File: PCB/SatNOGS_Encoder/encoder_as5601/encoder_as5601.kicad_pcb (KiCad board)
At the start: 2 copper layers, 25.4 x 25.4 mm, 12 parts, among them P1 CONN_02X05, Q1 Q_NMOS_GSD, U1 AS5601

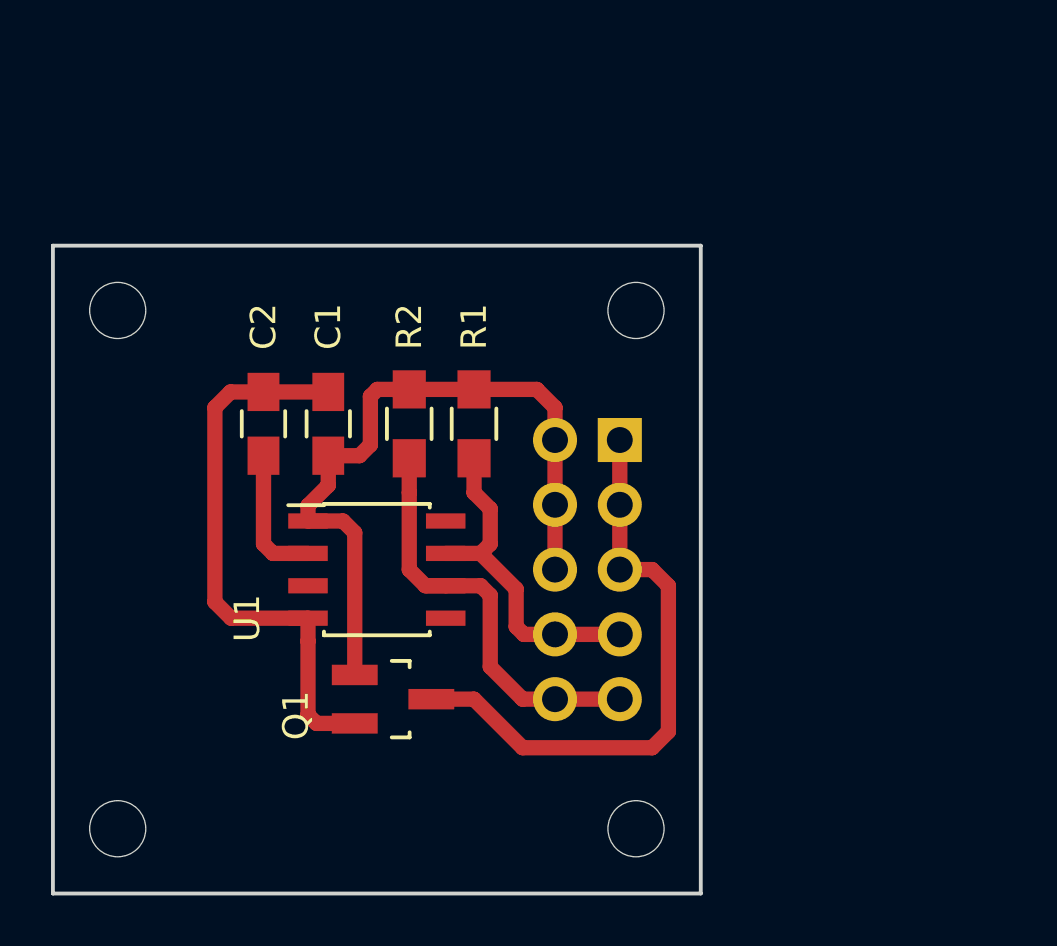
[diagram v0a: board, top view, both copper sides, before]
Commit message: wip
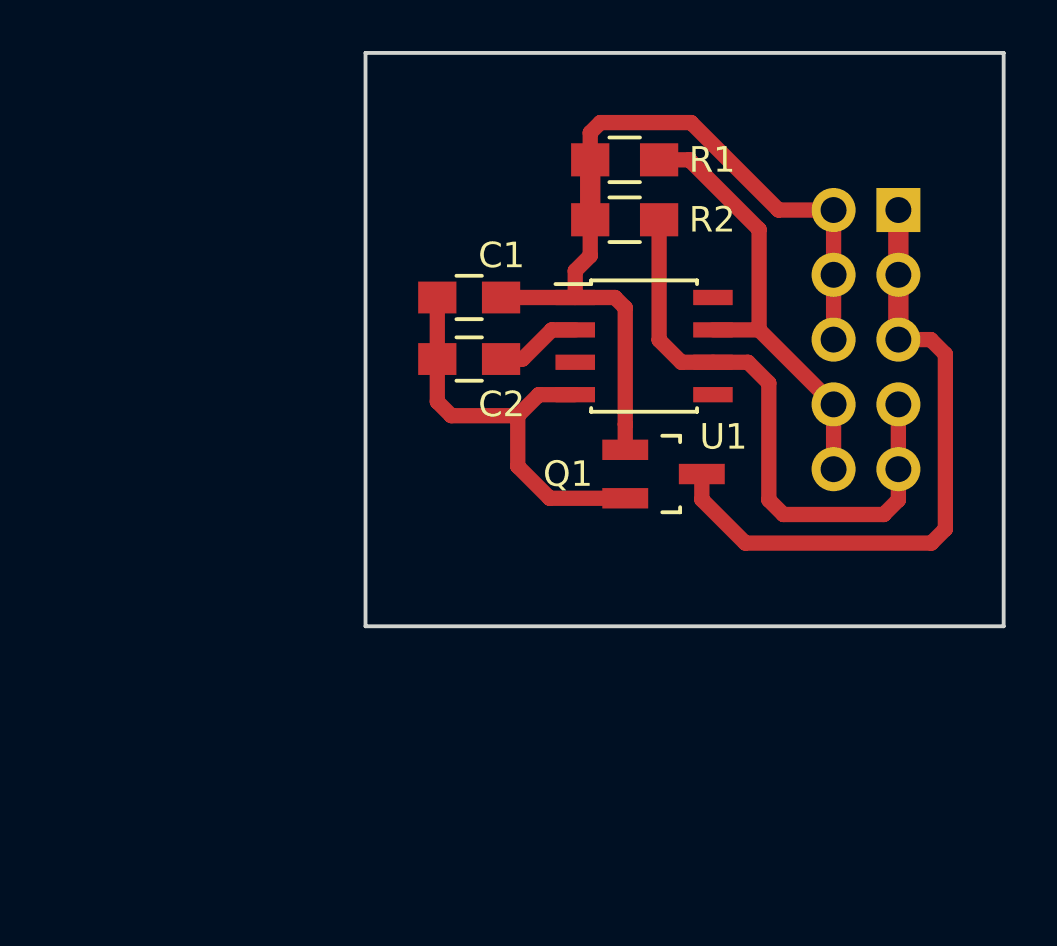
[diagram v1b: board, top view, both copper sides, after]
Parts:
- removed REF** (x4): MountingHole_2.2mm_M2, Mounting_Holes:MountingHole_2.2mm_M2
- removed ©2016 LSF: SatNOGS-Encoder, Symbols:OSHW-Logo2_7.3x6mm_SilkScreen
- added SatNOGS_Encoder: ©2016 Libre Space Foundation, Symbols:Symbol_OSHW-Logo_SilkScreen, B.Cu at (137.9, 79.3)
- moved P1 14.2 mm to (153.8, 74.8)
- moved Q1 13.8 mm to (144.6, 85.2)
- moved U1 13.7 mm to (143.8, 80.1)
- moved R1 11.9 mm to (143.1, 72.8), turned to 0 degrees
- moved R2 11.6 mm to (143.1, 75.2), turned to 0 degrees
- moved C2 8.46 mm to (137.0, 80.6), turned to 180 degrees
- moved C1 7.42 mm to (137.0, 78.2), turned to 180 degrees
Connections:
- P1 pad 10: /SDA -> /SCL
- P1 pad 7: /SCL -> /SDA
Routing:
- net /SDA: track 16.4 -> 23.6 mm
- net +5V: track 28.2 -> 33.5 mm
- net GND: track 22.0 -> 16.8 mm
- net /SCL: track 13.2 -> 17.5 mm
- net Net-(P1-Pad1): track 23.3 -> 25.5 mm
- net Net-(C2-Pad1): track 5.36 -> 3.38 mm
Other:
- board size 25.4 x 25.4 mm -> 25 x 22.5 mm
- net class power removed
- net class signals removed
- board text added: "SDA|SCL"
- board text removed: "SCL"
- board text removed: "SDA"
